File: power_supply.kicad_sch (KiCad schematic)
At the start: 18 parts, among them J1 Разъём к автомобилю 2x16 (32 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, U6 MC78M05CDTG, U7 AMS1117-3.3

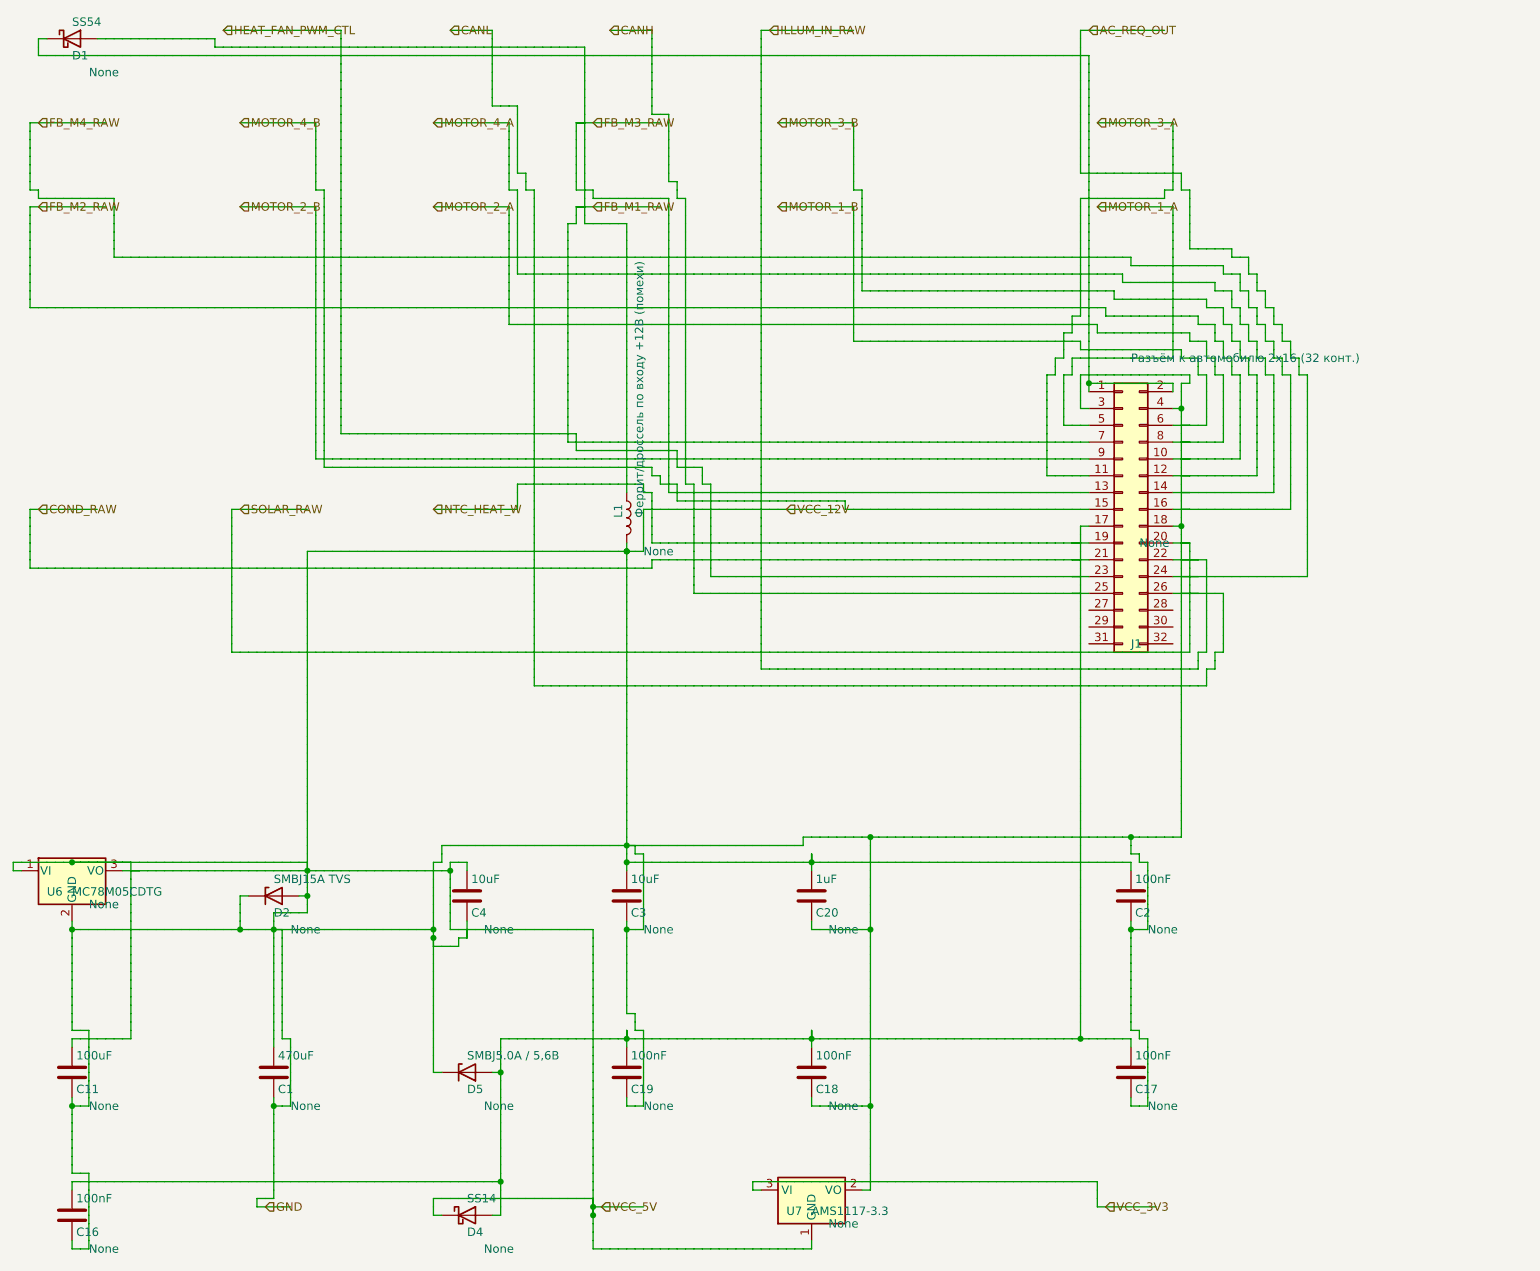
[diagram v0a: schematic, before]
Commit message: fix writer
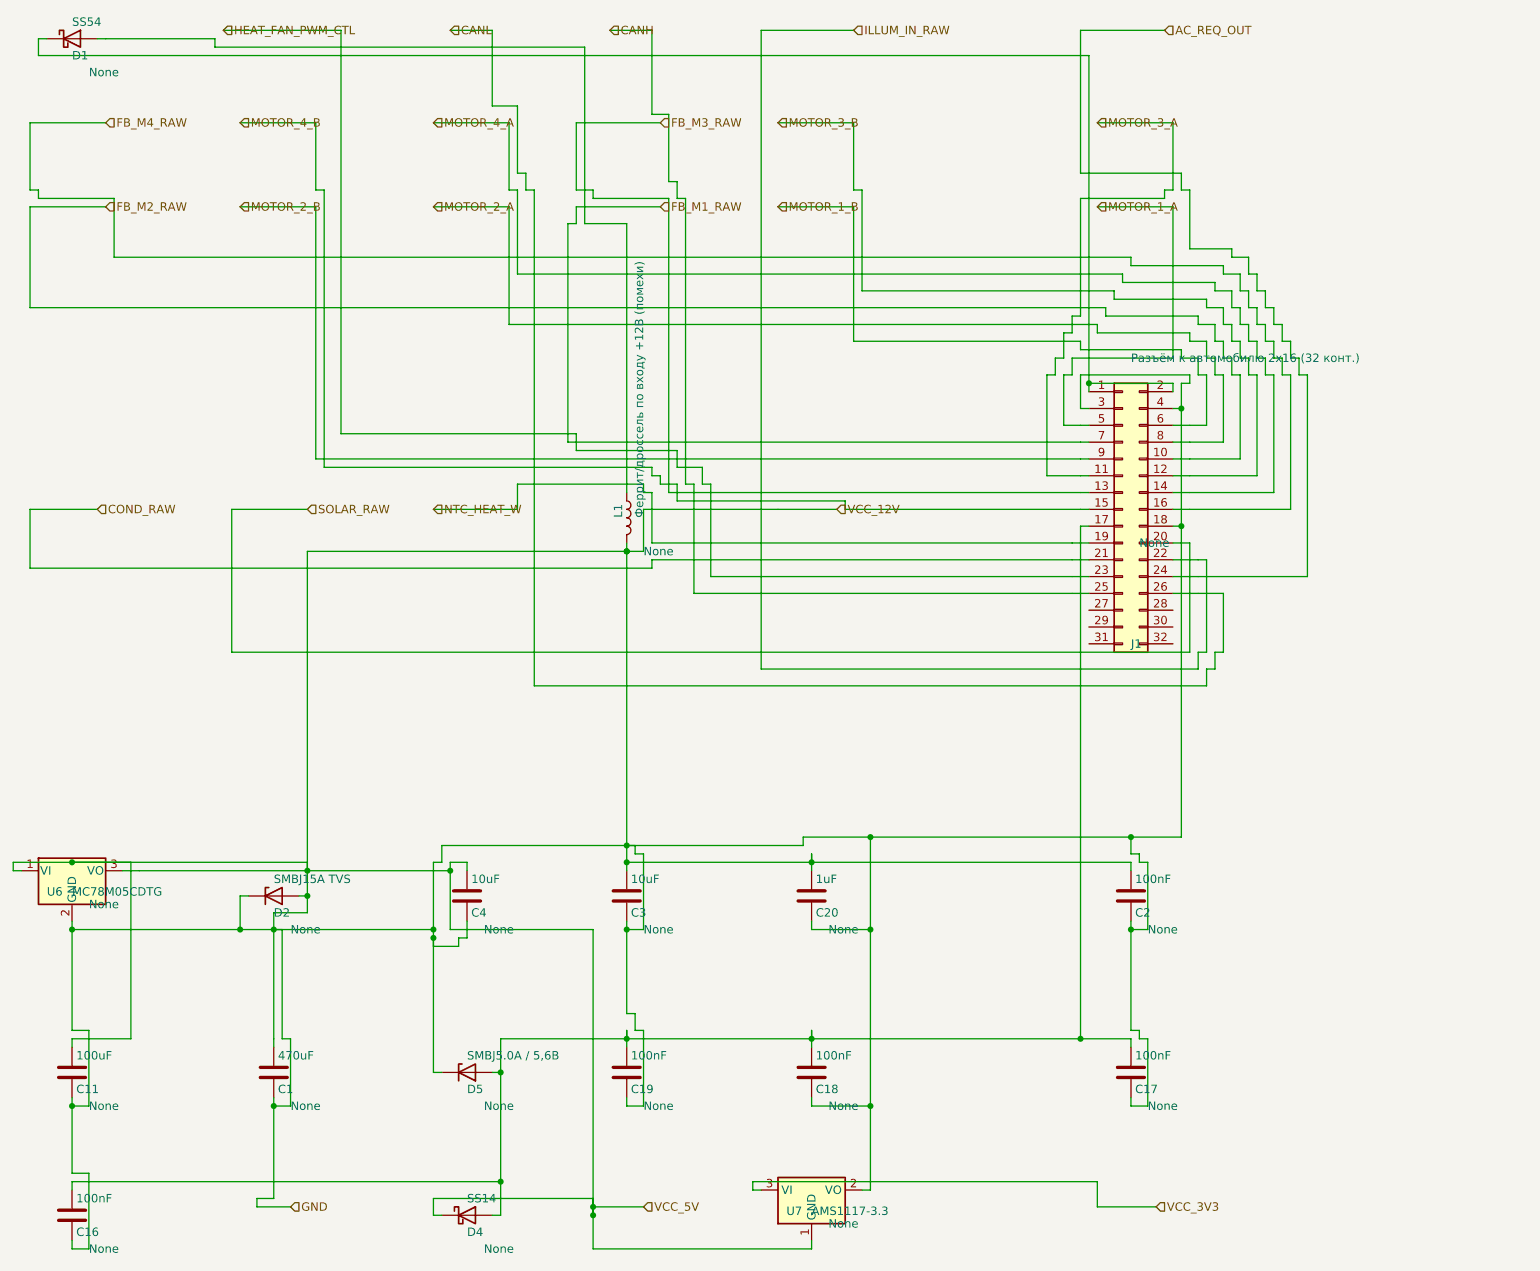
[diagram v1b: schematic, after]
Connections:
- net AC_REQ_OUT: no longer C1.1, C1.2, C11.1, C11.2, C16.1, C16.2, C17.1, C17.2, C18.1, C18.2, C19.1, C19.2, C2.1, C2.2, C20.1, C20.2, C3.1, C3.2, C4.1, C4.2, D1.1 (K), D1.2 (A), D2.1 (K), D2.2 (A), D4.1 (K), D4.2 (A), D5.1 (K), D5.2 (A), J1.1 (Pin_1), J1.10 (Pin_10), J1.11 (Pin_11), J1.12 (Pin_12), J1.13 (Pin_13), J1.14 (Pin_14), J1.15 (Pin_15), J1.16 (Pin_16), J1.17 (Pin_17), J1.18 (Pin_18), J1.19 (Pin_19), J1.2 (Pin_2), J1.20 (Pin_20), J1.21 (Pin_21), J1.22 (Pin_22), J1.23 (Pin_23), J1.25 (Pin_25), J1.26 (Pin_26), J1.3 (Pin_3), J1.4 (Pin_4), J1.5 (Pin_5), J1.6 (Pin_6), J1.7 (Pin_7), J1.8 (Pin_8), J1.9 (Pin_9), L1.1, L1.2, U6.1 (VI), U6.2 (GND), U6.3 (VO), U7.1 (GND), U7.2 (VO), U7.3 (VI)
- new net: C16.1, C17.1, C18.1, C19.1, D4.2 (A), D5.2 (A), J1.17 (Pin_17)
- new net: D1.2 (A), L1.1
- new net: D1.1 (K), J1.1 (Pin_1), J1.2 (Pin_2)
- new net CANH: J1.25 (Pin_25)
- new net CANL: J1.26 (Pin_26)
- new net COND_RAW: J1.21 (Pin_21)
- new net FB_M1_RAW: J1.7 (Pin_7)
- new net FB_M2_RAW: J1.10 (Pin_10)
- new net FB_M3_RAW: J1.13 (Pin_13)
- new net FB_M4_RAW: J1.16 (Pin_16)
- new net GND: C1.1, C1.2, C11.1, C11.2, C16.2, C17.2, C18.2, C19.2, C2.1, C2.2, C20.1, C20.2, C3.1, C3.2, C4.1, C4.2, D2.1 (K), D2.2 (A), D4.1 (K), D5.1 (K), J1.18 (Pin_18), J1.3 (Pin_3), J1.4 (Pin_4), L1.2, U6.1 (VI), U6.2 (GND), U6.3 (VO), U7.1 (GND), U7.2 (VO)
- new net HEAT_FAN_PWM_CTL: J1.23 (Pin_23)
- new net ILLUM_IN_RAW: J1.22 (Pin_22)
- new net MOTOR_1_A: J1.5 (Pin_5)
- new net MOTOR_1_B: J1.6 (Pin_6)
- new net MOTOR_2_A: J1.8 (Pin_8)
- new net MOTOR_2_B: J1.9 (Pin_9)
- new net MOTOR_3_A: J1.11 (Pin_11)
- new net MOTOR_3_B: J1.12 (Pin_12)
- new net MOTOR_4_A: J1.14 (Pin_14)
- new net MOTOR_4_B: J1.15 (Pin_15)
- new net NTC_HEAT_W: J1.19 (Pin_19)
- new net SOLAR_RAW: J1.20 (Pin_20)
- new net VCC_3V3: U7.3 (VI)
